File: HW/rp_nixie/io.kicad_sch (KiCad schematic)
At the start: 25 parts, among them J3 USB_C_Receptacle_USB2.0, SW2 +, SW3 OK, SW4 -

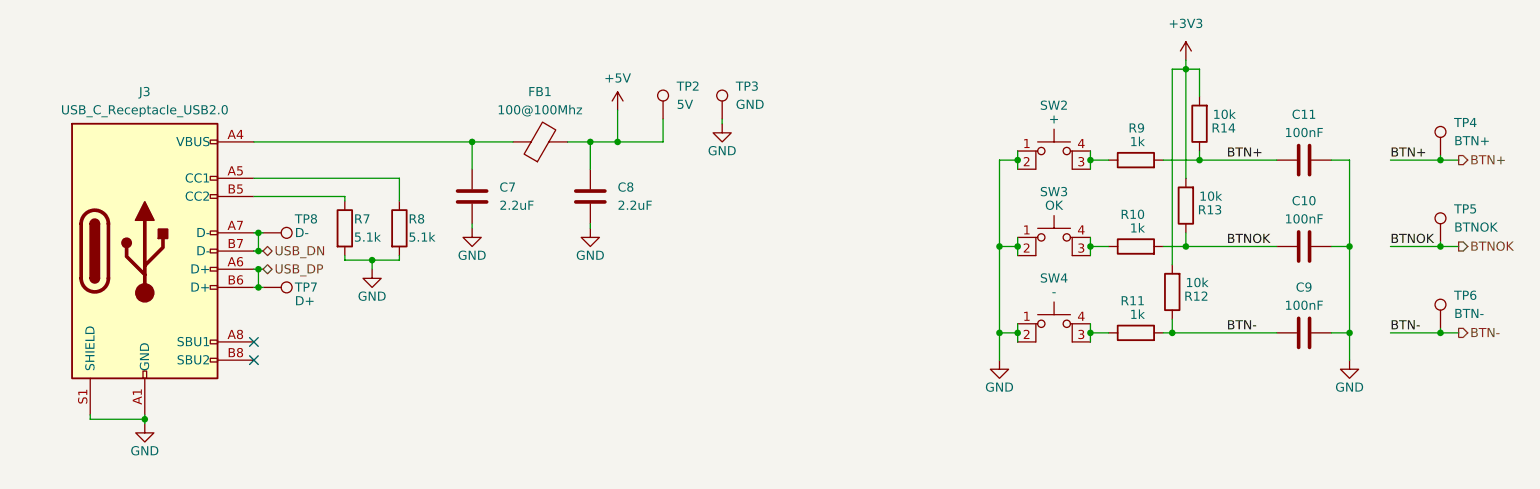
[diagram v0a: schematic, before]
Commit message: some schematic work
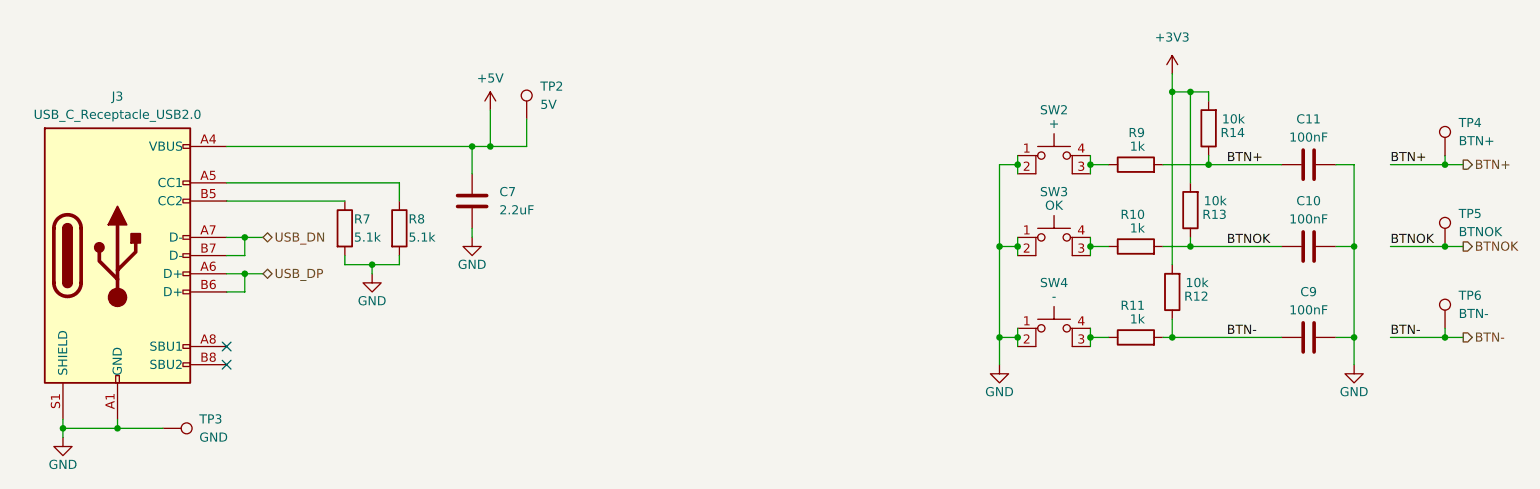
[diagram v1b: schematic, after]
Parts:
- removed C8: 2.2uF, symbol Device:C
- removed FB1: 100@100Mhz, symbol Device:FerriteBead
- removed TP7: D+, symbol Connector:TestPoint
- removed TP8: D-, symbol Connector:TestPoint
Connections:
- net +5V: now also C7.1, J3.A4 (VBUS), J3.A9 (VBUS), J3.B4 (VBUS), J3.B9 (VBUS)
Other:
- moved on the sheet: C10, C11, C7, C9, J3, R11, R13, R14, R9, SW2, SW4, TP2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
